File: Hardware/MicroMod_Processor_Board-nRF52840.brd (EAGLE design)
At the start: 22 x 22 mm, 30 parts, among them J2 MICROMOD-2222, U1 W25QXX128MBIT-6X5, U2 MDBT50Q, Y1 32.768kHz

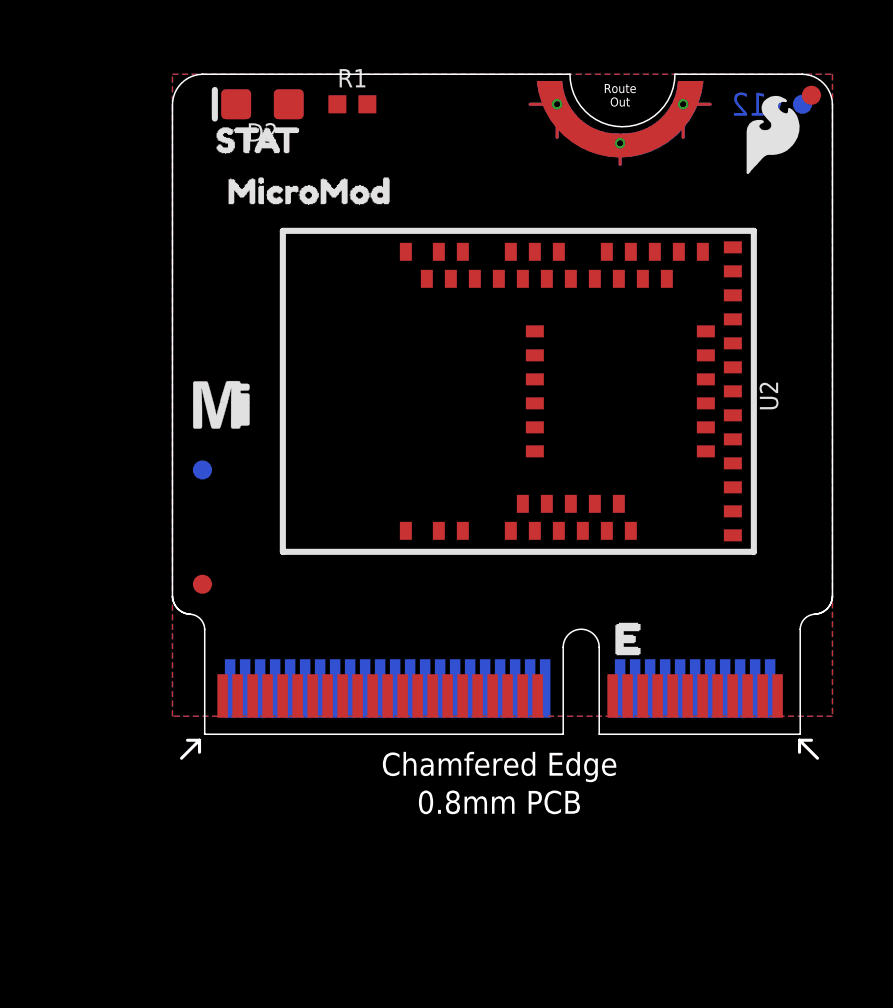
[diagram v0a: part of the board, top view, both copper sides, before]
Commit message: Finished preliminary schematic
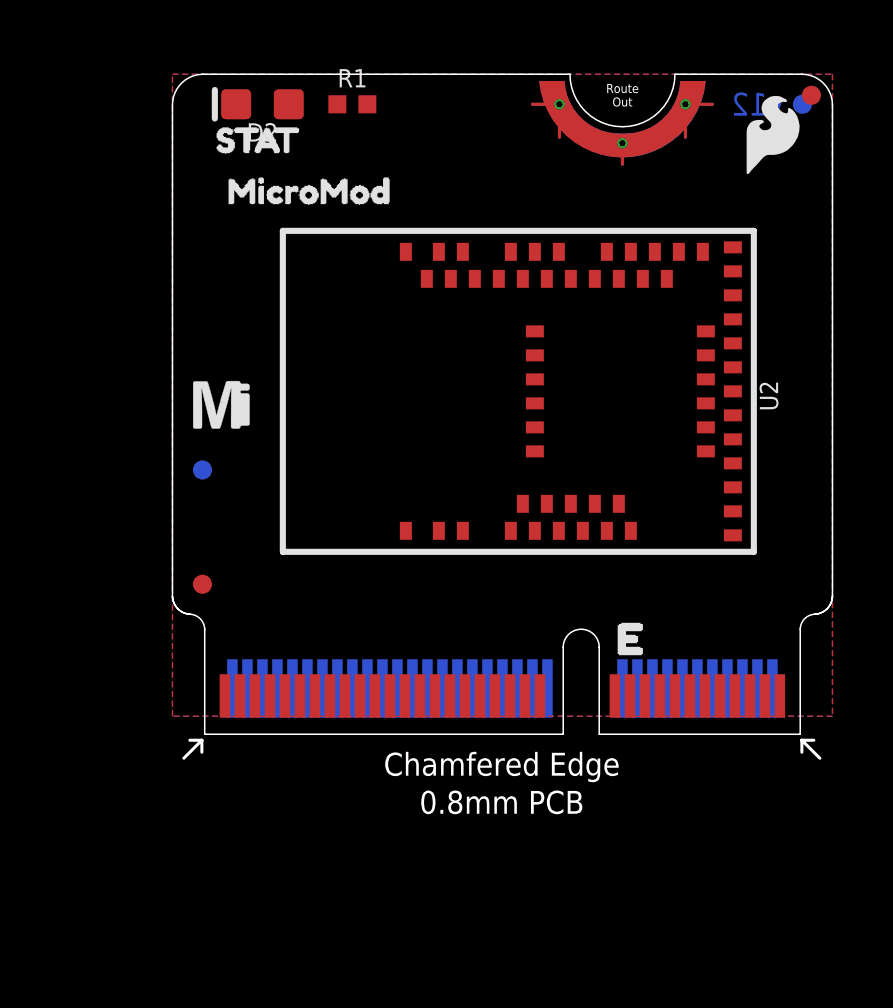
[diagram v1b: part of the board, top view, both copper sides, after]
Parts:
- moved J2 0.08 mm to (11.0, 0.00)
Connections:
- net PDM_DATA: now also U2.19; no longer U2.50
- net RTS1: now also U2.50; no longer U2.19

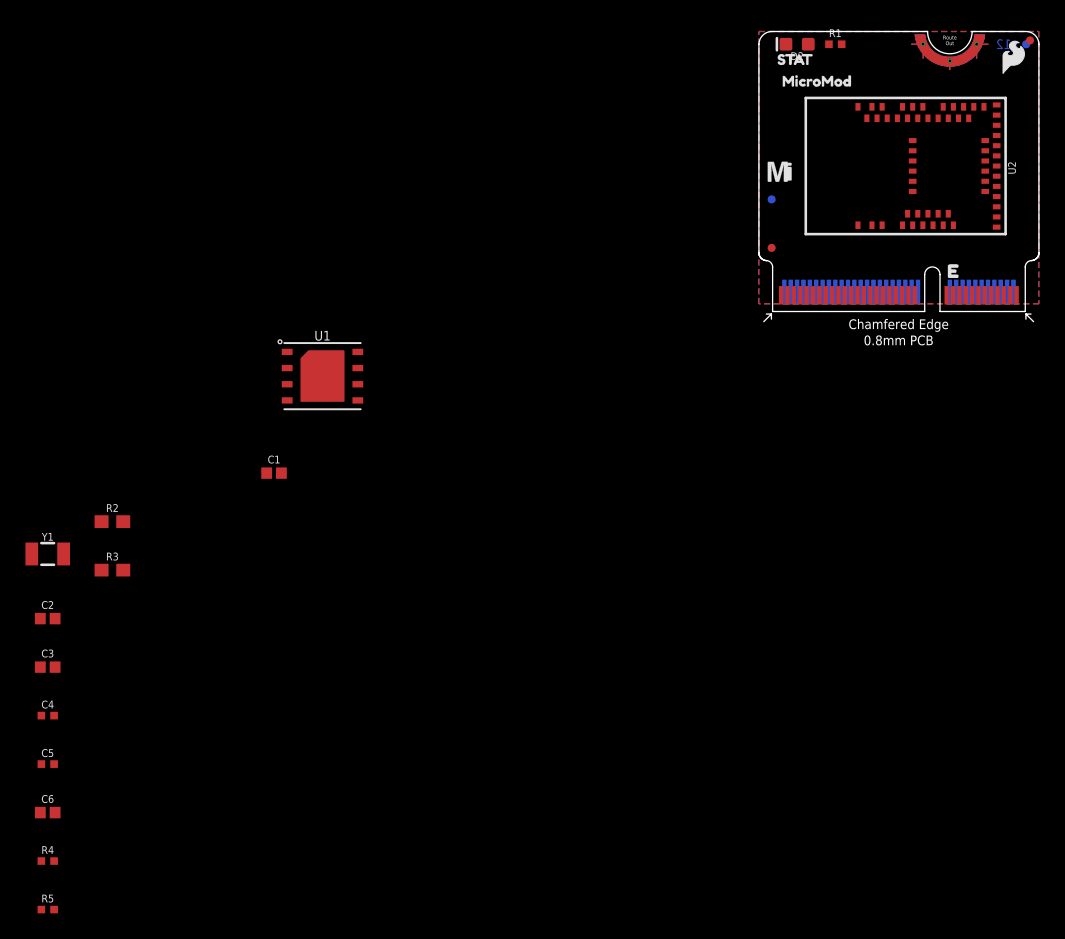
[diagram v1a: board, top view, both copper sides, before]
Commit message: Preliminary layout of PB
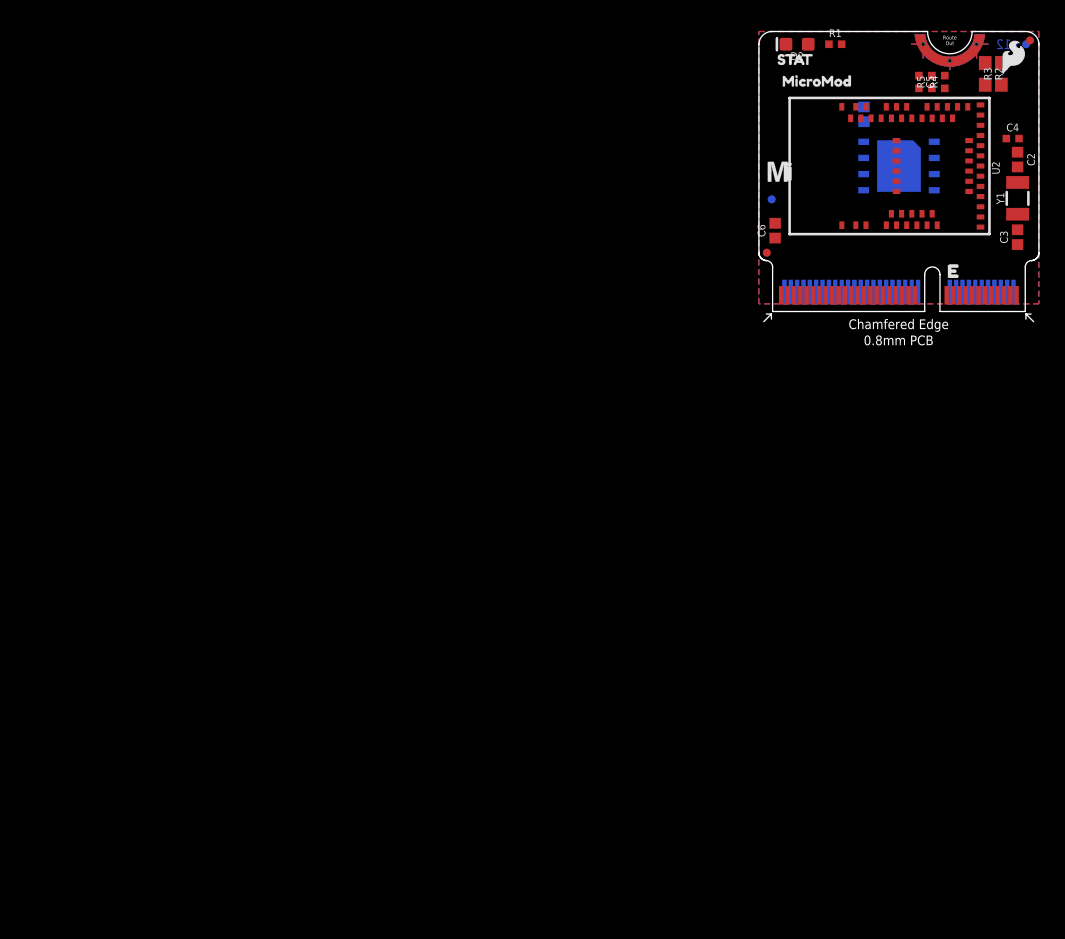
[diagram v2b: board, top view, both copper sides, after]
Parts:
- moved R5 95.2 mm to (13.6, 18.0), turned to 90 degrees
- moved R4 93.4 mm to (14.6, 18.0), turned to 90 degrees
- moved C4 88.3 mm to (19.9, 13.6)
- moved C5 86.9 mm to (12.6, 18.0), turned to 270 degrees
- moved C2 84.3 mm to (20.3, 11.9), turned to 270 degrees
- moved C3 83.4 mm to (20.3, 5.84), turned to 90 degrees
- moved Y1 81.2 mm to (20.3, 8.89), turned to 90 degrees
- moved R3 80.0 mm to (19.1, 18.7), turned to 90 degrees
- moved R2 77.1 mm to (17.8, 18.7), turned to 270 degrees
- moved C6 73.2 mm to (1.27, 6.35), turned to 90 degrees
- moved C1 54.3 mm to (8.26, 15.5), flipped to the bottom, turned to 90 degrees
- moved U1 48.2 mm to (11.0, 11.4), flipped to the bottom
- moved U2 1.27 mm to (10.2, 11.4)
- moved FD1 0.54 mm to (0.62, 4.62)
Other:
- board text removed: "N. Seidle"
